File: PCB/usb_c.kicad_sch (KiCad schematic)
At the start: 3 parts

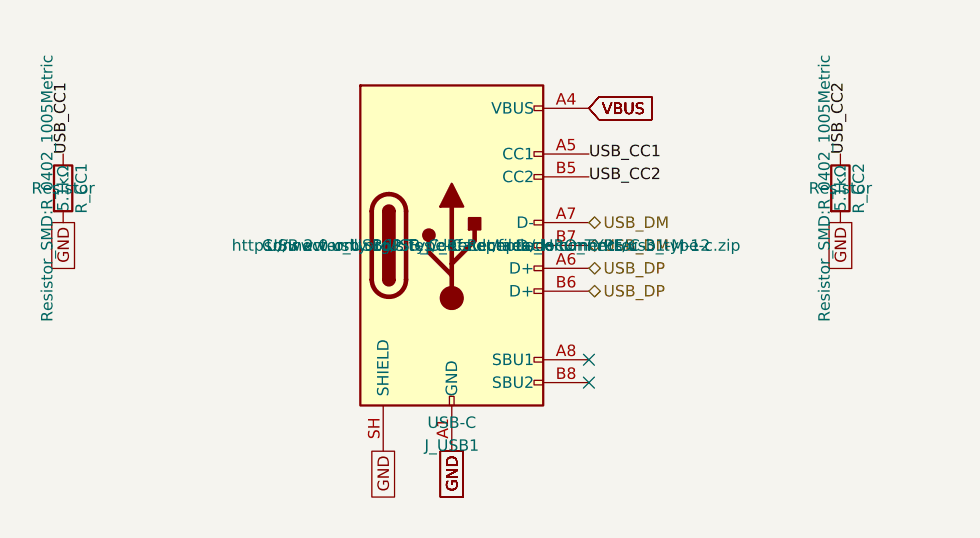
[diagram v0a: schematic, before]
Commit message: task: first validation pass
This is the results post first kicad-happy run.
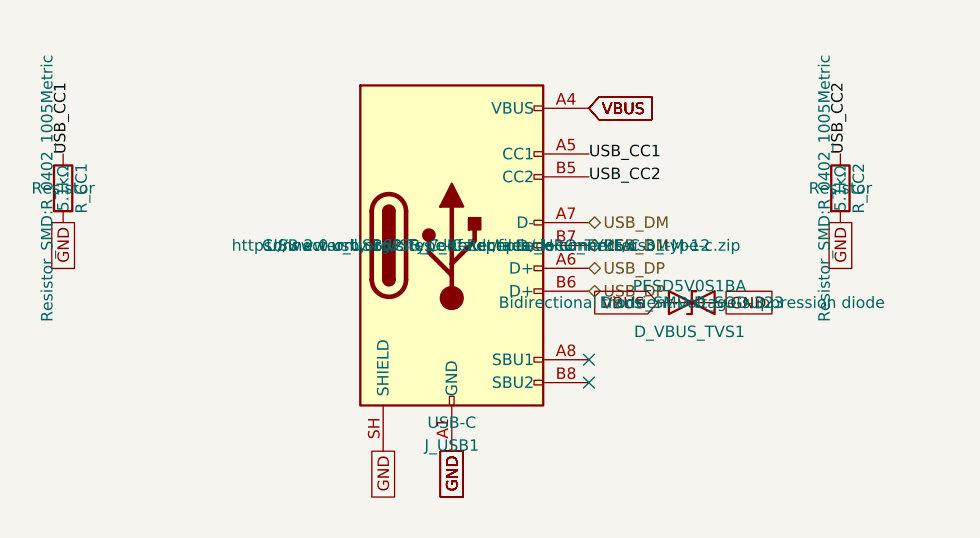
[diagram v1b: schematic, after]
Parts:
- added D_VBUS_TVS1: PESD5V0S1BA, Diode_SMD:D_SOD-323, symbol Device:D_TVS
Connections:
- net GND: now also D_VBUS_TVS1.2 (A2)
- net VBUS: now also D_VBUS_TVS1.1 (A1)
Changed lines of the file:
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@@
+		)
+	)
+	(global_label "GND"
+		(shape passive)
+		(at 179.07 114.3 0)
+		(fields_autoplaced yes)
+		(effects
+			(font
+				(size 1.27 1.27)
+			)
+			(justify left)
+		)
+		(property "Intersheetrefs" "${INTERSHEET_REFS}"
+			(at 179.07 114.3 0)
+			(hide yes)
+			(show_name no)
+			(do_not_autoplace no)
+			(effects
+				(font
+					(size 1.27 1.27)
+				)
+			)
 		)
 	)
@@
 		(property "Intersheetrefs" "${INTERSHEET_REFS}"
 			(at 163.83 92.71 0)
+			(hide yes)
+			(show_name no)
+			(do_not_autoplace no)
+			(effects
+				(font
+					(size 1.27 1.27)
+				)
+			)
+		)
+	)
+	(global_label "VBUS"
+		(shape input)
+		(at 171.45 114.3 180)
+		(fields_autoplaced yes)
+		(effects
+			(font
+				(size 1.27 1.27)
+			)
+			(justify right)
+		)
+		(property "Intersheetrefs" "${INTERSHEET_REFS}"
+			(at 171.45 114.3 0)
 			(hide yes)
 			(show_name no)
@@
 					(unit 1)
 				)
+			)
+		)
+	)
+	(symbol
+		(lib_id "Device:D_TVS")
+		(at 175.26 114.3 0)
+		(unit 1)
+		(body_style 1)
+		(exclude_from_sim no)
+		(in_bom yes)
+		(on_board yes)
+		(in_pos_files yes)
+		(dnp no)
+		(fields_autoplaced yes)
+		(property "Reference" "D_VBUS_TVS1"
+			(at 175 117.54 0)
+			(show_name no)
+			(do_not_autoplace no)
+			(effects
+				(font
+					(size 1.27 1.27)
+				)
+			)
+		)
+		(property "Value" "PESD5V0S1BA"
+			(at 175 112.46 0)
+			(show_name no)
+			(do_not_autoplace no)
+			(effects
+				(font
+					(size 1.27 1.27)
+				)
+			)
+		)
+		(property "Footprint" "Diode_SMD:D_SOD-323"
+			(at 175.26 114.3 0)
+			(show_name no)
+			(do_not_autoplace no)
+			(effects
+				(font
+					(size 1.27 1.27)
+				)
+			)
+		)
+		(property "Datasheet" ""
+			(at 175.26 114.3 0)
+			(show_name no)
+			(do_not_autoplace no)
+			(effects
+				(font
+					(size 1.27 1.27)
+				)
+			)
+		)
+		(property "Description" "Bidirectional transient-voltage-suppression diode"
+			(at 175.26 114.3 0)
+			(show_name no)
+			(do_not_autoplace no)
+			(effects
+				(font
+					(size 1.27 1.27)
+				)
+			)
+		)
+		(pin "1"
+		)
+		(pin "2"
+		)
+		(instances
+			(project "snips_controller"
+				(path "/21935953-32a0-46ad-8079-8177920c6978/a79dce81-618b-4a1c-ac71-81a6b4c28e48"
+					(reference "D_VBUS_TVS1")
+					(unit 1)
+				)
